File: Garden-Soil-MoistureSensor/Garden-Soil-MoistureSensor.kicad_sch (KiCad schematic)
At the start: 4 parts

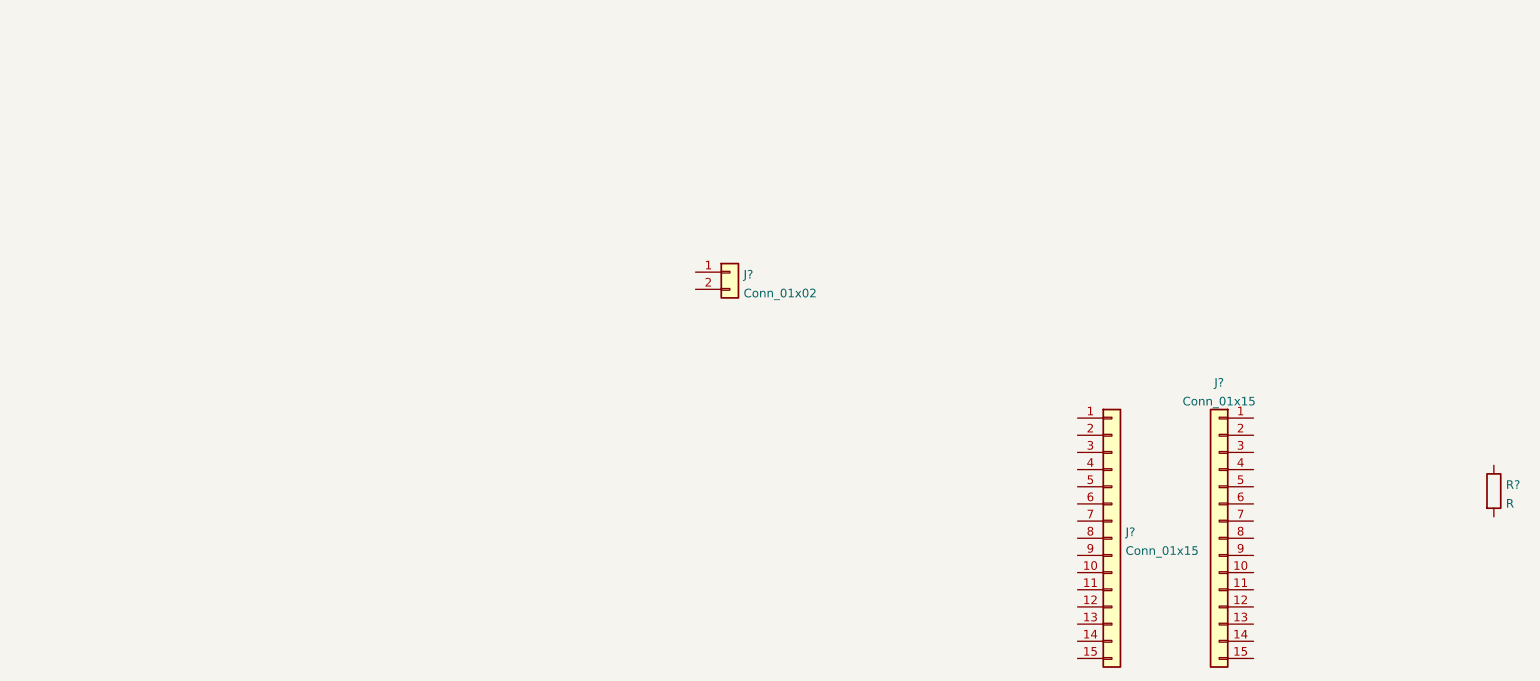
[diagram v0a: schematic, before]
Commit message: working on the PCB still selecting/designing things.
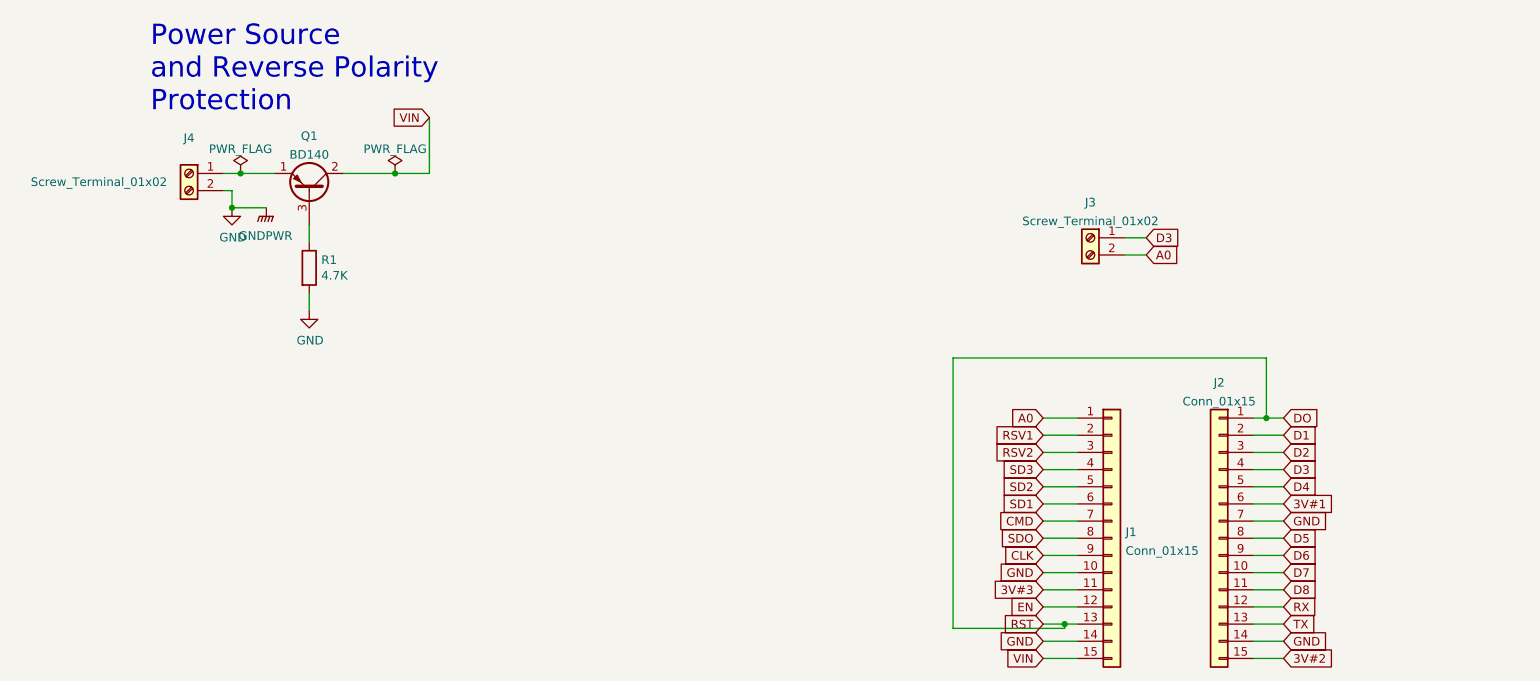
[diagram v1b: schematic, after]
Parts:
- removed J?: Conn_01x02, symbol Connector_Generic:Conn_01x02
- removed R?: R, symbol Device:R
- added J3, J4: Screw_Terminal_01x02, TerminalBlock_Phoenix:TerminalBlock_Phoenix_MKDS-1,5-2_1x02_P5.00mm_Horizontal, symbol Connector:Screw_Terminal_01x02
- added Q1: BD140, Package_TO_SOT_THT:TO-126-3_Vertical, symbol Transistor_BJT:BD140
- added R1: 4.7K, Resistor_THT:R_Axial_DIN0207_L6.3mm_D2.5mm_P2.54mm_Vertical, symbol Device:R
- J1, J2: renamed from J?; footprint (none) -> Connector_PinHeader_2.54mm:PinHeader_1x15_P2.54mm_Vertical
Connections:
- net DO: now reaches J2.1 (Pin_1)
- net DO: now also J1.13 (Pin_13)
- net D7: now reaches J2.10 (Pin_10)
- net D8: now reaches J2.11 (Pin_11)
- net RX: now reaches J2.12 (Pin_12)
- net TX: now reaches J2.13 (Pin_13)
- net GND: now reaches J2.14 (Pin_14)
- net GND: now also J1.10 (Pin_10), J1.14 (Pin_14), J2.7 (Pin_7), J4.2 (Pin_2), R1.2
- net 3V#2: now reaches J2.15 (Pin_15)
- net D1: now reaches J2.2 (Pin_2)
- net D2: now reaches J2.3 (Pin_3)
- net D3: now reaches J2.4 (Pin_4)
- net D3: now also J3.1 (Pin_1)
- net D4: now reaches J2.5 (Pin_5)
- net 3V#1: now reaches J2.6 (Pin_6)
- net D5: now reaches J2.8 (Pin_8)
- net D6: now reaches J2.9 (Pin_9)
- net A0: now reaches J1.1 (Pin_1)
- net A0: now also J3.2 (Pin_2)
- net 3V#3: now reaches J1.11 (Pin_11)
- net EN: now reaches J1.12 (Pin_12)
- net VIN: now reaches J1.15 (Pin_15)
- net VIN: now also Q1.2 (C)
- net RSV1: now reaches J1.2 (Pin_2)
- net RSV2: now reaches J1.3 (Pin_3)
- net SD3: now reaches J1.4 (Pin_4)
- net SD2: now reaches J1.5 (Pin_5)
- net SD1: now reaches J1.6 (Pin_6)
- net CMD: now reaches J1.7 (Pin_7)
- net SDO: now reaches J1.8 (Pin_8)
- net CLK: now reaches J1.9 (Pin_9)
- new net: J4.1 (Pin_1), Q1.1 (E)
- new net: Q1.3 (B), R1.1
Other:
- note added: "Power Source and Reverse Polarity Protection"
